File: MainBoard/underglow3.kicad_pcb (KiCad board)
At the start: 4 copper layers, 81.2 x 100.2 mm, 242 parts, among them J202 TC2030-IDC, J203 Micro_SD_Card_Det1, J301 Delphi_Sicma_24, J302 USB_A, J404 USB_B_Mini, K301 G6K-2F-Y DC12, Q301 AO3419, Q302 SI2302-TP, Q303 SI2302-TP, Q304 AO3419, Q305 SI2302-TP, Q306 SI2302-TP, Q307 AO3419, Q308 MMBT5551, Q309 SI2302-TP, Q310 SI2302-TP, Q311 SI2302-TP, Q312 MMBT5551, Q319 SI2302-TP, Q320 SI2302-TP, Q321 SI2302-TP, U201 T113-S3, U202 W25Q32JVSS, U203 ATECC608A-MAHDA, U301 SCT2650STER, U302 USBLC6-2SC6, U303 USBLC6-2SC6, U304 MCP1416T-E/OT, U305 MCP1416T-E/OT, U306 MCP1416T-E/OT, U307 MCP1416T-E/OT, U308 MCP1416T-E/OT, U309 MCP1416T-E/OT, U401 AP6212, U402 SY8088IAAC, U403 SY8088IAAC, U405 SN65HVD230, Y201 24Mhz, Y401 26Mhz

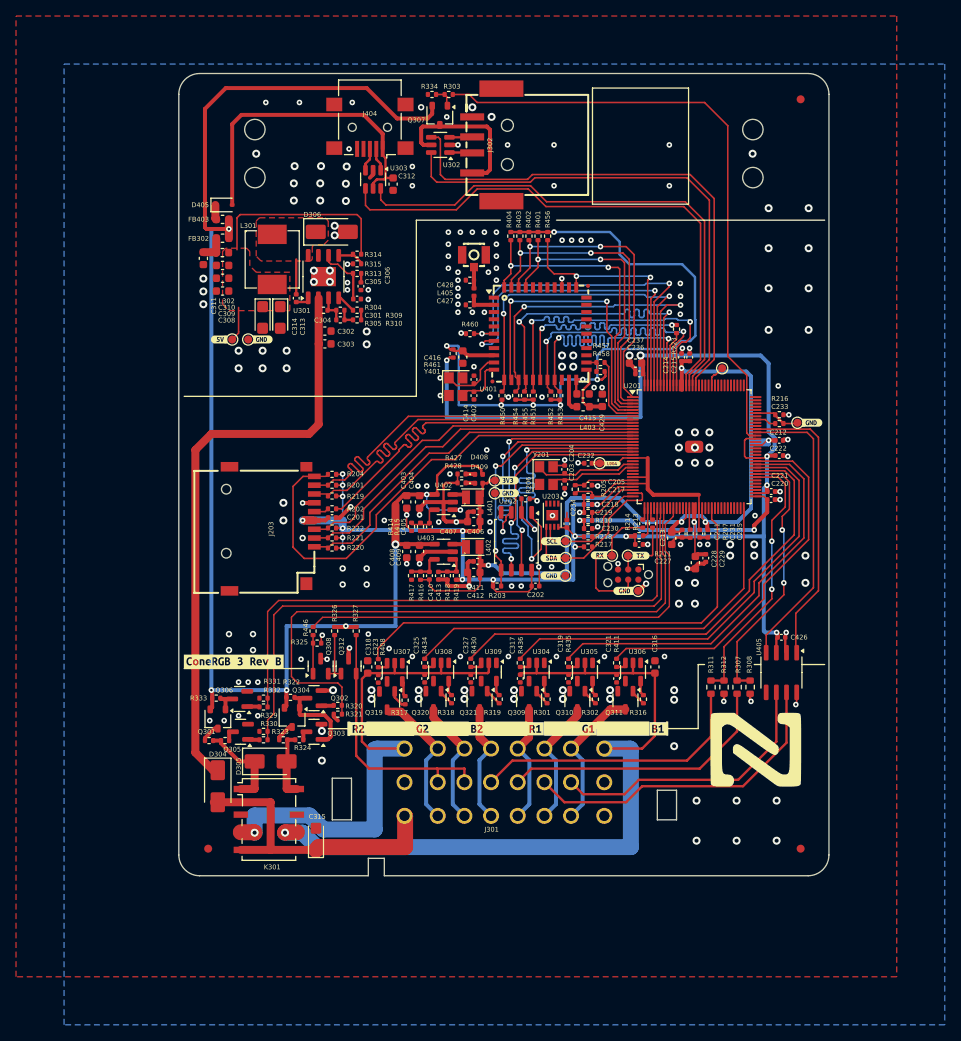
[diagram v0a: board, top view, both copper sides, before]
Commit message: Submit for production
Signed-off-by: Connor Rigby <connorr@hey.com>
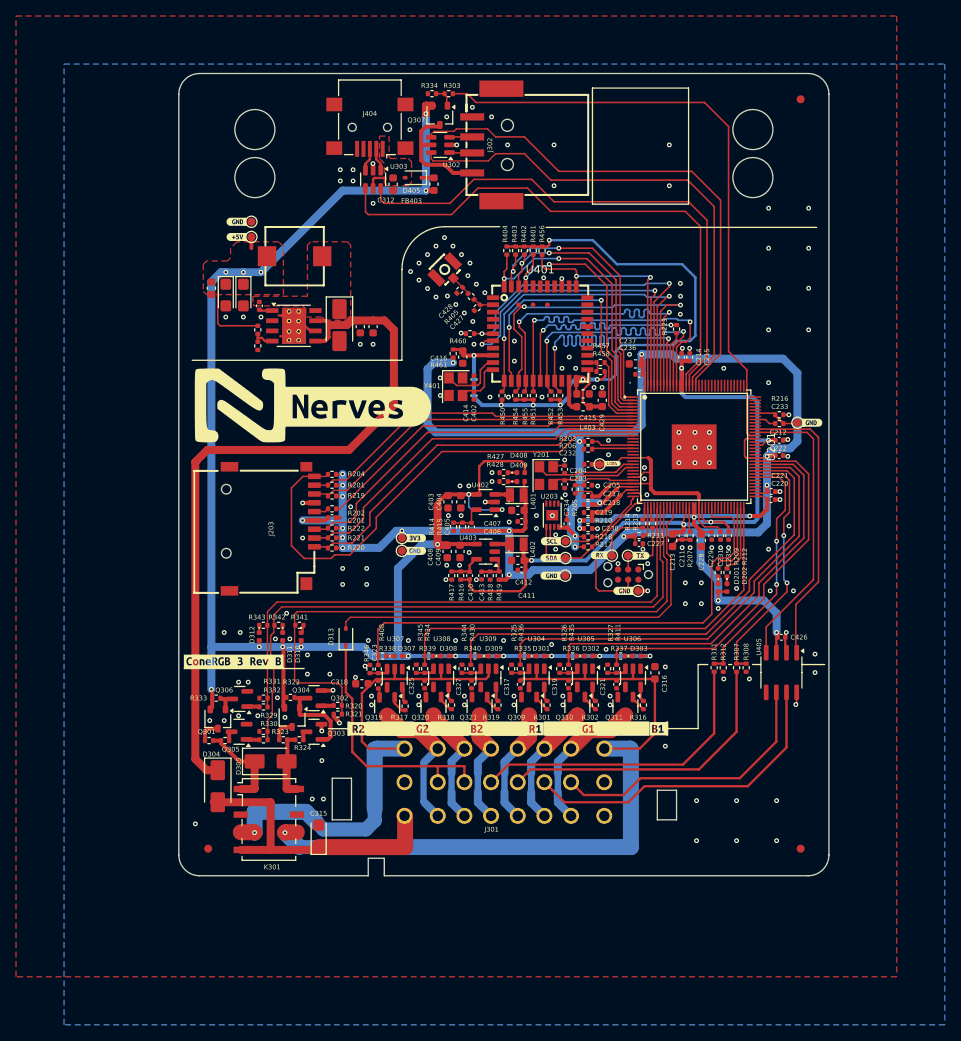
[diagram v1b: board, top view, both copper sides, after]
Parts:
- removed C202: 100nf, Capacitor_SMD:C_0402_1005Metric
- removed C301: 1uF, Resistor_SMD:R_0402_1005Metric
- removed C305: 22pF, Capacitor_SMD:C_0402_1005Metric
- removed C306: 3.3nF, Capacitor_SMD:C_0402_1005Metric
- removed C308: 10uF, Capacitor_SMD:C_0603_1608Metric
- removed C309: 220nF, Capacitor_SMD:C_0603_1608Metric
- removed C310: 68pF, Capacitor_SMD:C_0603_1608Metric
- removed FB302: 450mΩ ±25% 600Ω@100MHz, Inductor_SMD:L_0603_1608Metric
- removed L301: 8.2uH 3.7A, Inductor_LCSC:IND-SMD_L7.0-W6.6_FXL0630
- removed L302: 2.2uH, Inductor_SMD:L_0603_1608Metric
- removed L405: 0R, Inductor_SMD:L_0402_1005Metric
- removed Q308, Q312: MMBT5551, Package_TO_SOT_SMD:SOT-23
- removed R304, R305: 0R, Resistor_SMD:R_0402_1005Metric
- removed R309, R310, R314: 100k 1%, Resistor_SMD:R_0402_1005Metric
- removed R313: 33k 1%, Resistor_SMD:R_0402_1005Metric
- removed R315: 18.7k 1%, Resistor_SMD:R_0402_1005Metric
- removed R446: 1k, Resistor_SMD:R_0402_1005Metric
- removed TP201: TVIN, TestPoint:TestPoint_Pad_D1.0mm
- removed U202: W25Q32JVSS, Package_SO:SOIC-8_5.23x5.23mm_P1.27mm
- removed U301: SCT2650STER, Package_SO:HSOP-8-1EP_3.9x4.9mm_P1.27mm_EP2.41x3.1mm
- removed kibuzzard-65FE521F: G***, kibuzzard-65FE521F
- removed the kibuzzard-65FE522B at (85.1, 102.5)
- added D201: LED, LED_SMD:LED_0402_1005Metric, F.Cu at (142.1, 133.5)
- added D202: LED, LED_SMD:LED_0402_1005Metric, F.Cu at (143.2, 133.5)
- added D301: LED, LED_SMD:LED_0402_1005Metric, F.Cu at (119.9, 142.0)
- added D302: LED, LED_SMD:LED_0402_1005Metric, F.Cu at (125.9, 142.0)
- added D303: LED, LED_SMD:LED_0402_1005Metric, F.Cu at (131.9, 142.0)
- added D307: LED, LED_SMD:LED_0402_1005Metric, F.Cu at (102.2, 142.0)
- added D308: LED, LED_SMD:LED_0402_1005Metric, F.Cu at (108.0, 142.0)
- added D309: LED, LED_SMD:LED_0402_1005Metric, F.Cu at (113.9, 142.0)
- added D310: LED, LED_SMD:LED_0402_1005Metric, F.Cu at (90.0, 139.6)
- added D311: LED, LED_SMD:LED_0402_1005Metric, F.Cu at (87.7, 139.6)
- added D312: LED, LED_SMD:LED_0402_1005Metric, F.Cu at (84.8, 139.6)
- added D313: NSR0320MW2T1G, Diode_SMD:D_SOD-323, F.Cu at (95.6, 139.6)
- added L303: 4.7uH, easyeda2kicad:IND-SMD_L7.3-W7.3, F.Cu at (89.2, 92.1)
- added R209: 1k, Resistor_SMD:R_0402_1005Metric, F.Cu at (142.1, 131.6)
- added R212: 1k, Resistor_SMD:R_0402_1005Metric, F.Cu at (143.2, 131.6)
- added R335: 1k, Resistor_SMD:R_0402_1005Metric, F.Cu at (117.9, 142.0)
- added R336: 1k, Resistor_SMD:R_0402_1005Metric, F.Cu at (123.9, 142.0)
- added R337: 1k, Resistor_SMD:R_0402_1005Metric, F.Cu at (129.9, 142.0)
- added R338: 1k, Resistor_SMD:R_0402_1005Metric, F.Cu at (100.2, 142.0)
- added R339: 1k, Resistor_SMD:R_0402_1005Metric, F.Cu at (106.0, 142.0)
- added R340: 1k, Resistor_SMD:R_0402_1005Metric, F.Cu at (111.7, 142.0)
- added R341: 1k, Resistor_SMD:R_0402_1005Metric, F.Cu at (89.8, 138.2)
- added R342: 1k, Resistor_SMD:R_0402_1005Metric, F.Cu at (87.2, 138.2)
- added R343: 1k, Resistor_SMD:R_0402_1005Metric, F.Cu at (85.3, 138.2)
- added R344: 100k 1%, Resistor_SMD:R_0402_1005Metric, F.Cu at (110.1, 143.6)
- added R345: 100k 1%, Resistor_SMD:R_0402_1005Metric, F.Cu at (104.4, 143.6)
- added R346: 100k 1%, Resistor_SMD:R_0402_1005Metric, F.Cu at (98.6, 143.6)
- added R347: 10k, Resistor_SMD:R_0402_1005Metric, F.Cu at (84.6, 101.3)
- added R348: 3.3k, Resistor_SMD:R_0402_1005Metric, F.Cu at (84.6, 103.3)
- added R405: 0R, Resistor_SMD:R_0402_1005Metric, F.Cu at (111.2, 97.1)
- added U310: TPS5430DDA, Package_SO:TI_SO-PowerPAD-8_ThermalVias, F.Cu at (89.1, 100.8)
- added kibuzzard-6669C582: G***, kibuzzard-6669C582, F.Cu at (82.0, 89.7)
- added kibuzzard-6669C587: G***, kibuzzard-6669C587, F.Cu at (82.0, 87.8)
- added kibuzzard-666C6B51: G***, kibuzzard-666C6B51, F.Cu at (97.1, 110.9)
- K301: value G6K-2F-Y DC12 -> G6K-2F-Y-TR DC3
- R307, R311: footprint Resistor_SMD:R_0603_1608Metric -> Resistor_SMD:R_0402_1005Metric
- R308, R312: value 2.2k -> 3.9k; footprint Resistor_SMD:R_0603_1608Metric -> Resistor_SMD:R_0402_1005Metric
- R326, R327: value 1k -> 100k 1%
- U201: footprint Package_QFP:LQFP-128_14x14mm_P0.4mm -> CPU_Allwinner_T113-S3:LQFP-128_L14.0-W14.0-P0.40-LS16.0-BL-EP5.6
- U302, U303: value USBLC6-2SC6 -> SRV05-4
- U401: value AP6212 -> RL-SM02BD-8723BS; footprint Module_WiFi_BT:RL-SM02BD(RTL8723BS) -> Module_WiFi_BT:QFN-44_L12.0-W12.0-P0.90-TL_AP6212
- moved G*** 77.4 mm to (82.4, 110.7)
- moved R327 31.8 mm to (128.3, 143.6)
- moved R326 28.5 mm to (122.3, 143.6)
- moved FB403 26.8 mm to (106.6, 83.1), turned to -90 degrees
- moved R325 24.5 mm to (116.3, 143.6), turned to -90 degrees
- moved D405 23.9 mm to (104.0, 82.3), turned to 180 degrees
- moved R203 21.3 mm to (125.8, 115.2)
- moved TP302 14.7 mm to (83.8, 87.8), turned to 180 degrees
- moved TP303 13.7 mm to (102.6, 127.3)
- moved kibuzzard-65FEF020 13.7 mm to (104.3, 127.3)
- moved TP304 13.7 mm to (102.6, 128.9)
- moved kibuzzard-65FE522B 13.7 mm to (104.3, 128.9)
- moved TP301 13.0 mm to (83.8, 89.7), turned to 180 degrees
- moved D306 11.7 mm to (94.8, 100.7), turned to -90 degrees
- moved R206 9.97 mm to (125.8, 116.2), turned to 180 degrees
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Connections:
- net /Power/SW renamed /Power/PH
- C304 pad 1: Net-(U301-BOOT) -> /Power/BOOT
- C311 pad 1: Net-(C311-Pad1) -> +5V
- C313 pad 1: Net-(C308-Pad1) -> +5V
- C314 pad 1: Net-(C308-Pad1) -> +5V
- J302 pad 2: Net-(J302-D-) -> /Power/USB1_DN
- J302 pad 3: Net-(J302-D+) -> /Power/USB1_DP
- J302 pad 6: (no net) -> unconnected-(J302-Shield-Pad5)
- J404 pad 2: Net-(J404-D-) -> /Power/USB0_DN
- J404 pad 3: Net-(J404-D+) -> /Power/USB0_DP
- R325 pad 1: Net-(Q308-B) -> GND
- R325 pad 2: GND -> Net-(U304-IN)
- R326 pad 1: +5V -> GND
- R326 pad 2: Net-(Q308-E) -> Net-(U305-IN)
- R327 pad 1: +5V -> GND
- R327 pad 2: /Power/LEDC_OUT -> Net-(U306-IN)
- R401 pad 2: /Application/HCI_RTS -> /Application/HCI_CTS
- R402 pad 2: /Application/HCI_TX -> /Application/HCI_RX
- R403 pad 2: /Application/HCI_RX -> /Application/HCI_TX
- R404 pad 1: /Application/HCI_CTS -> /Application/HCI_RTS
- TP301 pad 1: Net-(C308-Pad1) -> +5V
- U201 pad 107: Net-(U201-VCC-TVIN) -> unconnected-(U201-VCC-TVIN-Pad107)
- U201 pad 112: /Application/USB1_DP -> /Power/USB1_DP
- U201 pad 113: /Application/USB1_DN -> /Power/USB1_DN
- U201 pad 114: /Application/USB0_DN -> /Power/USB0_DN
- U201 pad 115: /Application/USB0_DP -> /Power/USB0_DP
- U201 pad 62: unconnected-(U201-PD7-Pad62) -> /Application/LED_ST1
- U201 pad 63: unconnected-(U201-PD8-Pad63) -> /Application/LED_ST2
- U302 pad 1: Net-(J302-D-) -> /Power/USB1_DN
- U302 pad 3: Net-(J302-D+) -> /Power/USB1_DP
- U302 pad 4: /Application/USB1_DP -> /Power/USB1_DP
- U302 pad 6: /Application/USB1_DN -> /Power/USB1_DN
- U303 pad 1: Net-(J404-D-) -> /Power/USB0_DN
- U303 pad 3: Net-(J404-D+) -> /Power/USB0_DP
- U303 pad 4: /Application/USB0_DP -> /Power/USB0_DP
- U303 pad 6: /Application/USB0_DN -> /Power/USB0_DN
- U401 pad 41: /Application/HCI_RTS -> /Application/HCI_CTS
- U401 pad 42: /Application/HCI_TX -> /Application/HCI_RX
- U401 pad 43: /Application/HCI_RX -> /Application/HCI_TX
- U401 pad 44: /Application/HCI_CTS -> /Application/HCI_RTS
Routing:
- net /Power/USB0_DP: track 0.00 -> 71.8 mm
- net /Power/USB0_DN: track 0.00 -> 70.2 mm
- net /Application/USB0_DP: track 68.1 -> 0.00 mm
- net /Power/USB1_DP: track 0.00 -> 67.8 mm
- net /Application/USB0_DN: track 66.3 -> 0.00 mm
- net /Application/USB1_DP: track 65.9 -> 0.00 mm
- net /Power/USB1_DN: track 0.00 -> 65.7 mm
- net /Application/USB1_DN: track 63.4 -> 0.00 mm
- net GND: track 86.1 -> 36.0 mm, vias 221 -> 197
- net +5V: track 192.6 -> 229.4 mm, vias 7 -> 18
- net /Power/VBUS: track 38.5 -> 2.81 mm
- net /Application/SPI0_CLK: track 34.5 -> 0.00 mm, vias 2 -> 0
- net /Application/SPI0_WP: track 34.3 -> 0.00 mm, vias 2 -> 0
- net /Application/SPI0_CS0: track 34.0 -> 0.00 mm, vias 2 -> 0
- net /Application/SPI0_HLD: track 32.4 -> 0.00 mm, vias 2 -> 0
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- added copper zone on F.Cu, net +5V
- added copper zone on F.Cu, net /Power/VBUS
- removed copper zone on F.Cu, net Net-(C308-Pad1)
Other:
- outline, holes or cut-outs redrawn

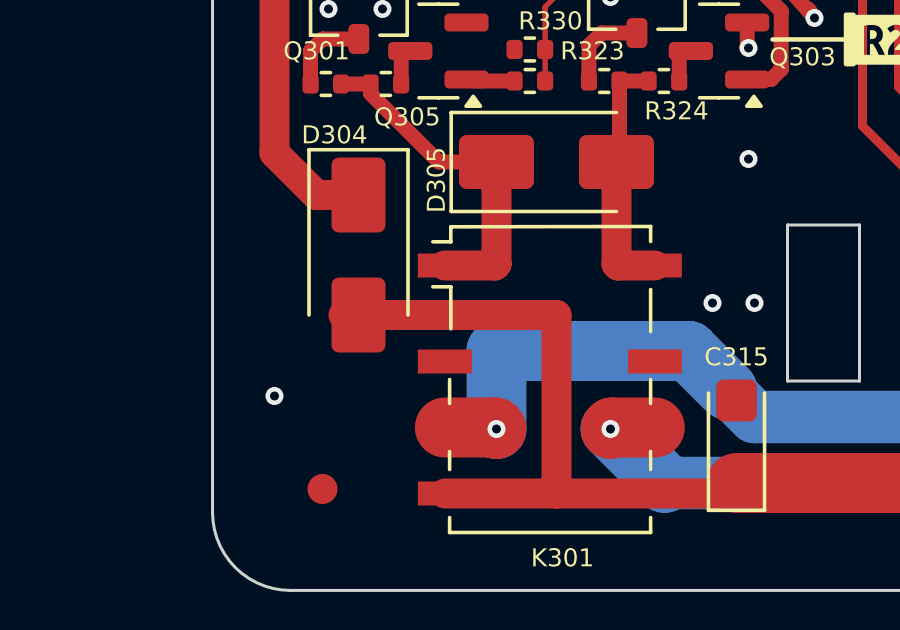
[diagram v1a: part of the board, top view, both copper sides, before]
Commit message: Doc updates
Signed-off-by: Connor Rigby <connorr@hey.com>
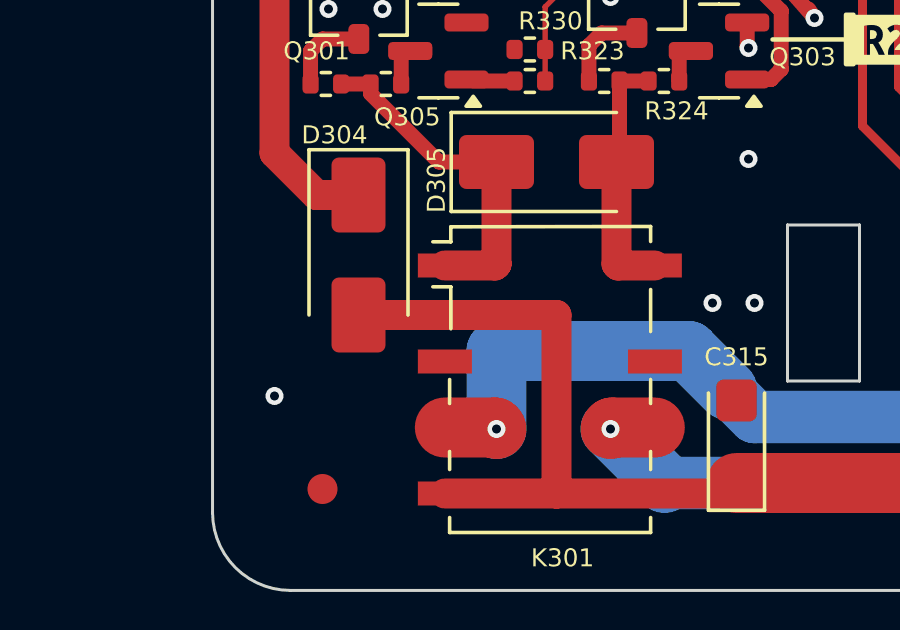
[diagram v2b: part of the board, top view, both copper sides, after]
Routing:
- net /Power/VIN: track 37.2 -> 36.7 mm
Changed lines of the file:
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@@
 			(pintype "passive+no_connect")
 		)
-		(model "C:/Users/konno/Desktop/workspace/connorrigby/underglow3/library/work/JLC2KiCad_lib/footprint/packages3d/USB-A-SMD_USB-234-BCW.step"
+		(model "${KIPRJMOD}/../library/work/JLC2KiCad_lib/footprint/packages3d/USB-A-SMD_USB-234-BCW.step"
 			(offset
 				(xyz 0 -5.000066 4.000001)
@@
 			)
 		)
-		(model "C:/Users/konno/Desktop/workspace/connorrigby/underglow3/library/Connector_LCSC_USB.pretty/packages3d/mini_usb_wifi_adapter.stp"
+		(model "${KIPRJMOD}/../library/Connector_LCSC_USB.pretty/packages3d/mini_usb_wifi_adapter.stp"
 			(offset
 				(xyz 0 -15 4)
@@
 	)
 	(segment
-		(start 86.2 160.270254)
-		(end 79.1 160.270254)
-		(width 1)
+		(start 103 165.870254)
+		(end 92.2 165.870254)
+		(width 2)
 		(layer "F.Cu")
 		(net 34)
 	)
 	(segment
-		(start 103 165.870254)
-		(end 92.2 165.870254)
-		(width 2)
+		(start 86.2 160.270254)
+		(end 79.6 160.270254)
+		(width 1)
 		(layer "F.Cu")
 		(net 34)
@@
 	(segment
 		(start 86.2 166.220254)
+		(end 86.2 160.270254)
+		(width 1)
+		(layer "F.Cu")
+		(net 34)
+	)
+	(segment
+		(start 86.2 166.220254)
 		(end 82.4775 166.220254)
 		(width 1)
@@
 		(width 1)
 		(layer "F.Cu")
-		(net 34)
-	)
-	(segment
-		(start 86.2 166.220254)
-		(end 86.2 160.270254)
-		(width 1)
-		(layer "F.Cu")
